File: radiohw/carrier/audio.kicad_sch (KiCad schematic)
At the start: 3 parts, among them U4 PCM2902, U5 PCM2902

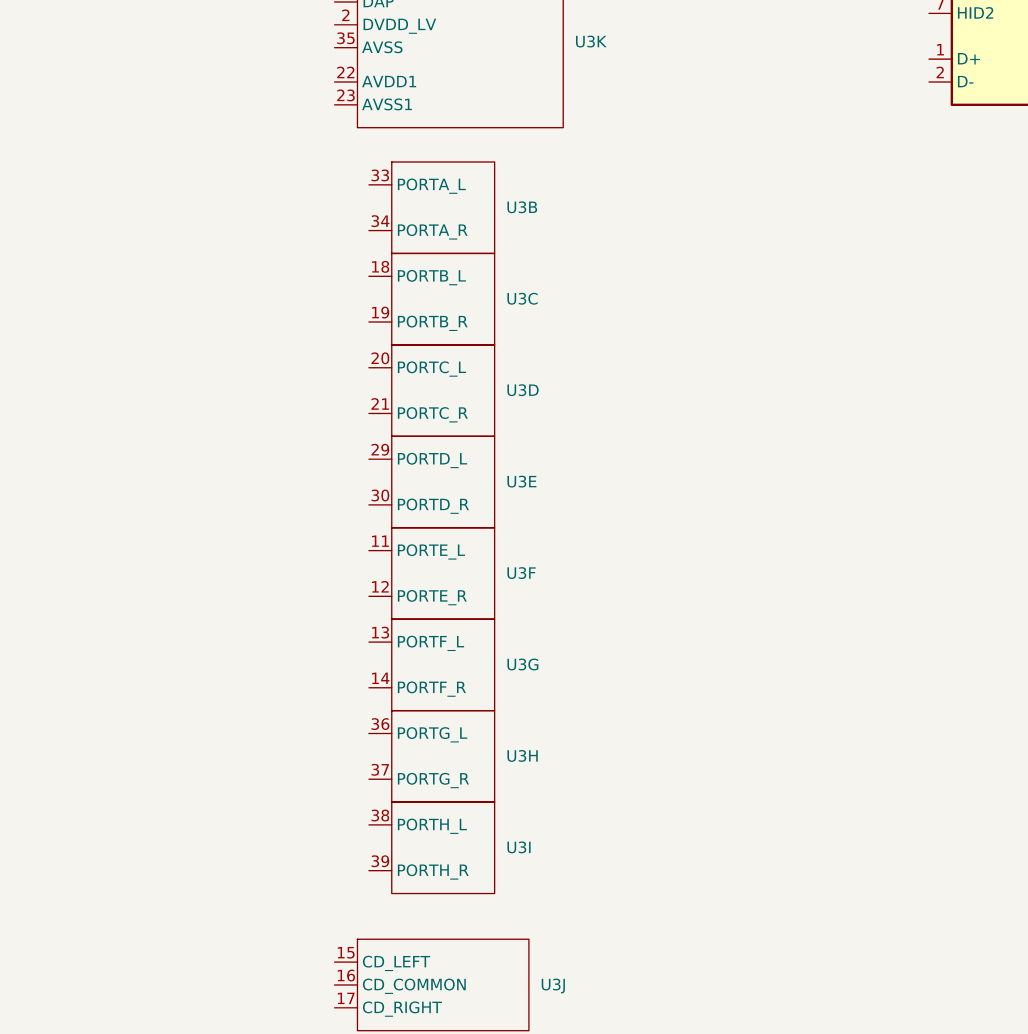
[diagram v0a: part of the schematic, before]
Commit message: Schematic development.
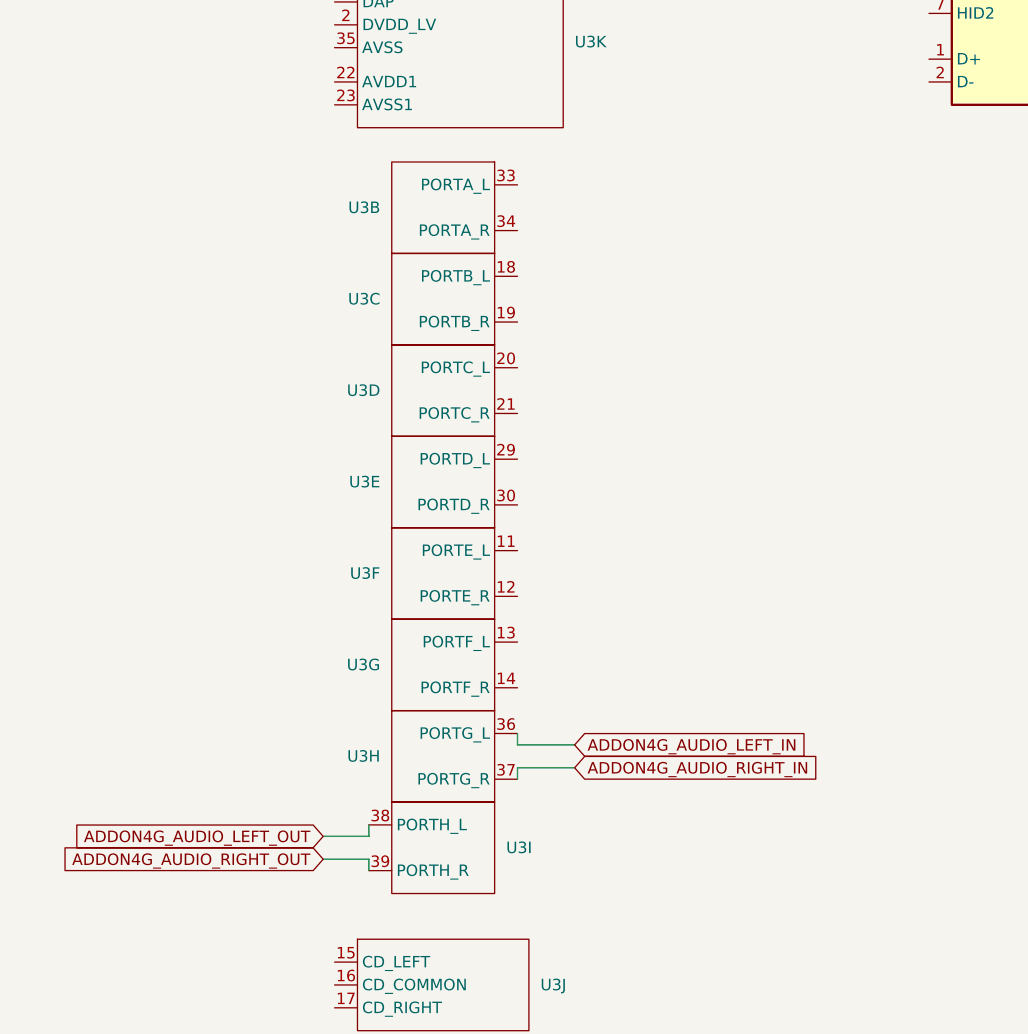
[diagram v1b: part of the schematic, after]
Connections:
- net ADDON4G_AUDIO_LEFT_OUT: now reaches U3.38 (PORTH_L)
- net ADDON4G_AUDIO_RIGHT_OUT: now reaches U3.39 (PORTH_R)
- net ADDON4G_AUDIO_LEFT_IN: now reaches U3.36 (PORTG_L)
- net ADDON4G_AUDIO_RIGHT_IN: now reaches U3.37 (PORTG_R)
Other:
- moved on the sheet: U3B, U3C, U3D, U3E, U3F, U3G, U3H

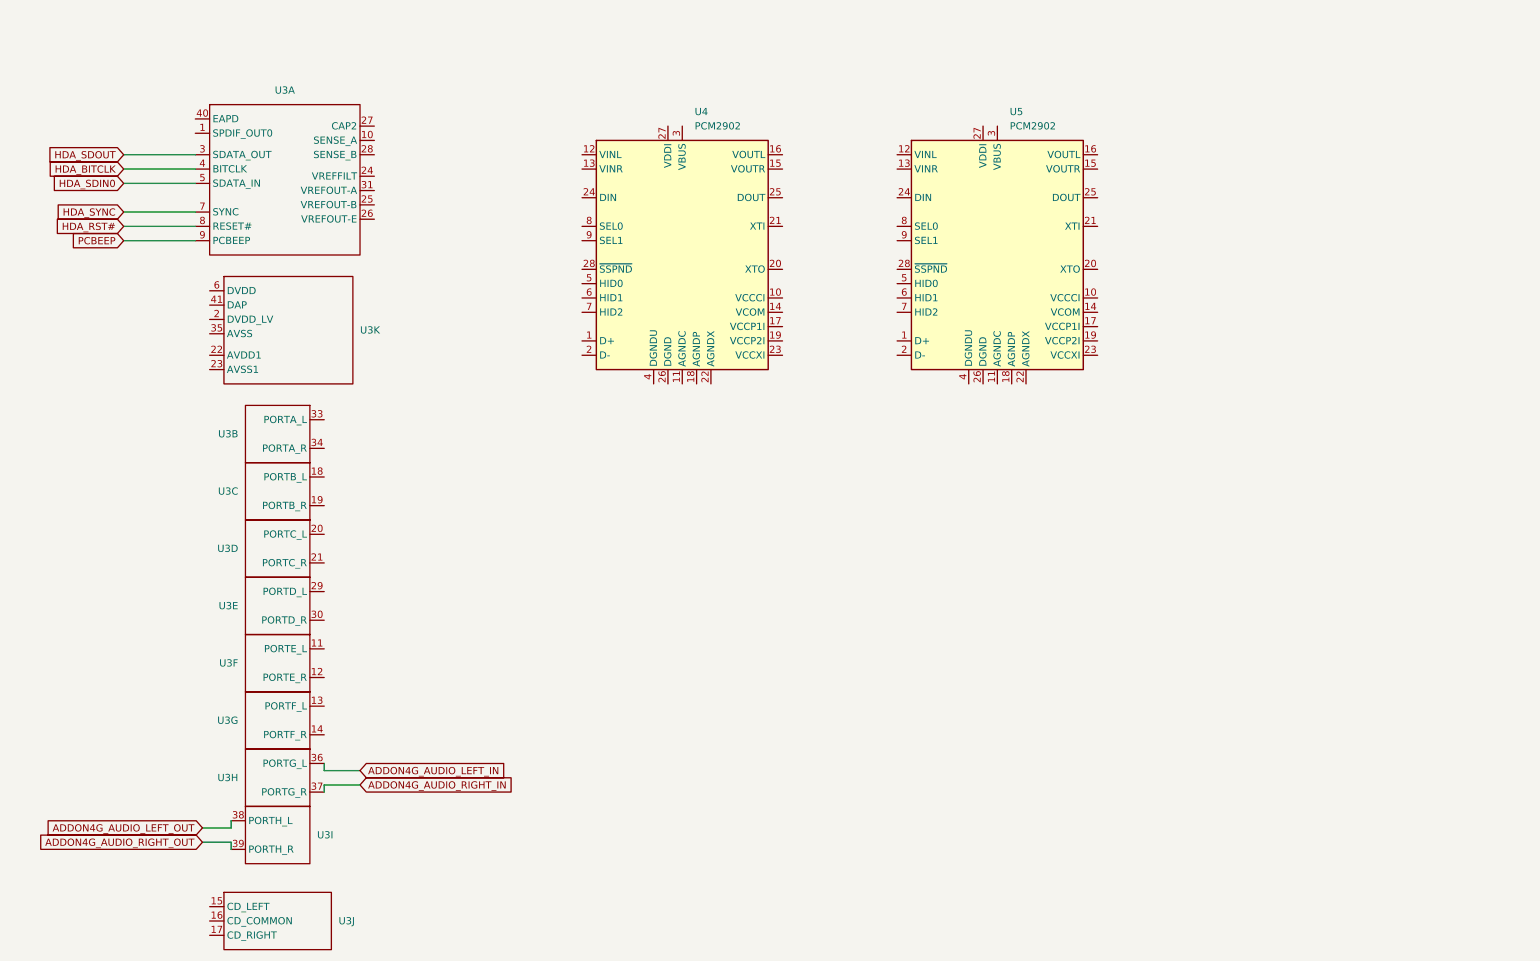
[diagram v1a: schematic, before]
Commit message: Schematic work.
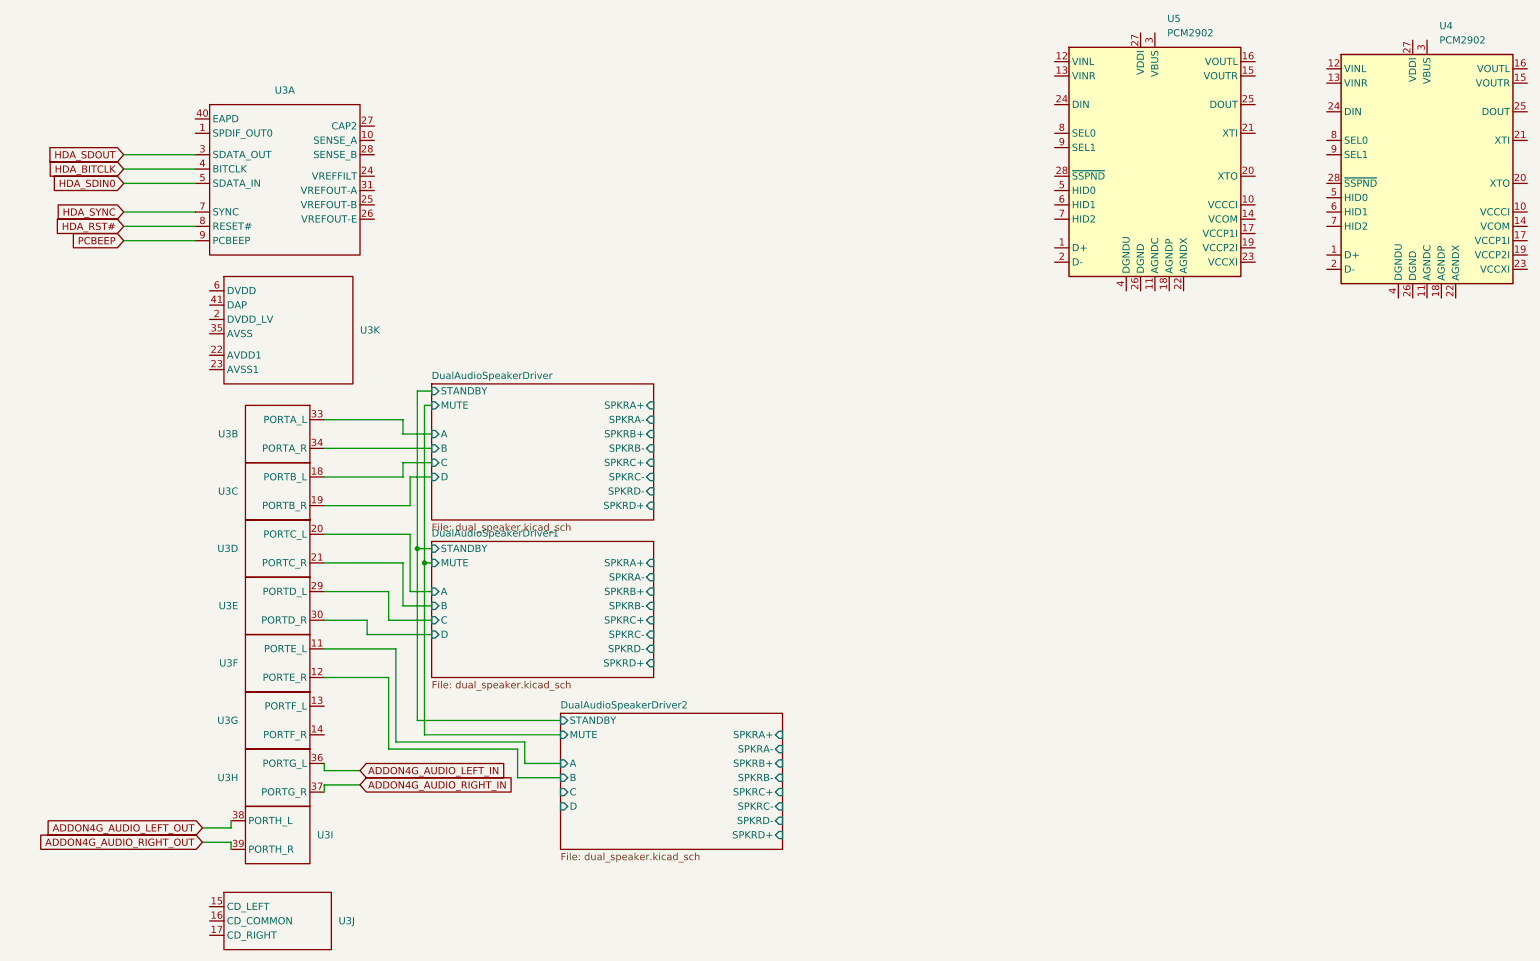
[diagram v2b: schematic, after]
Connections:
- net DualAudioSpeakerDriver1/C: now reaches U3.29 (PORTD_L)
- net DualAudioSpeakerDriver1/D: now reaches U3.30 (PORTD_R)
- net DualAudioSpeakerDriver2/A: now reaches U3.11 (PORTE_L)
- net DualAudioSpeakerDriver2/B: now reaches U3.12 (PORTE_R)
- net DualAudioSpeakerDriver/A: now reaches U3.33 (PORTA_L)
- net DualAudioSpeakerDriver/B: now reaches U3.34 (PORTA_R)
- net DualAudioSpeakerDriver1/A: now reaches U3.20 (PORTC_L)
- net DualAudioSpeakerDriver1/B: now reaches U3.21 (PORTC_R)
- net DualAudioSpeakerDriver/C: now reaches U3.18 (PORTB_L)
- net DualAudioSpeakerDriver/D: now reaches U3.19 (PORTB_R)
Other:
- added sheet DualAudioSpeakerDriver (dual_speaker.kicad_sch)
- added sheet DualAudioSpeakerDriver1 (dual_speaker.kicad_sch)
- added sheet DualAudioSpeakerDriver2 (dual_speaker.kicad_sch)
- moved on the sheet: U4, U5

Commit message: Audio schematic development.
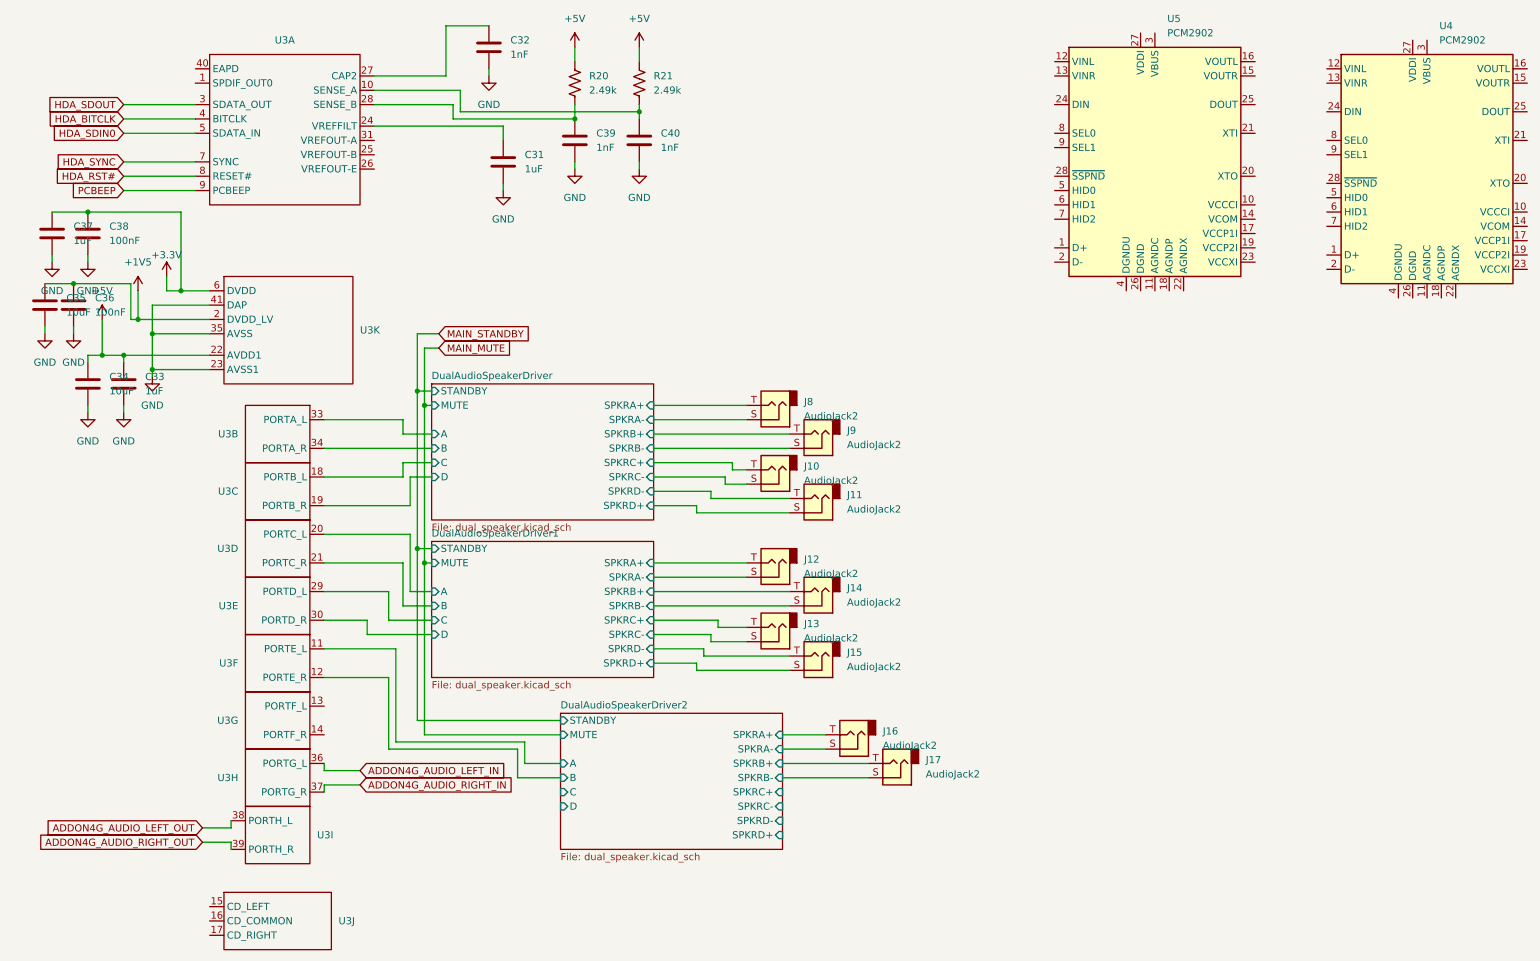
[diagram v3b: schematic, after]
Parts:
- added C31, C33, C37: 1uF, Capacitor_SMD:C_0805_2012Metric_Pad1.18x1.45mm_HandSolder, symbol Device:C
- added C32, C39, C40: 1nF, Capacitor_SMD:C_0402_1005Metric_Pad0.74x0.62mm_HandSolder, symbol Device:C
- added C34, C35: 10uF, symbol Device:C
- added C36, C38: 100nF, Capacitor_SMD:C_0603_1608Metric_Pad1.08x0.95mm_HandSolder, symbol Device:C
- added J10, J11, J12, J13, J14, J15, J16, J17, J8, J9: AudioJack2, symbol Connector_Audio:AudioJack2
- added R20, R21: 2.49k, Capacitor_SMD:C_0603_1608Metric_Pad1.08x0.95mm_HandSolder, symbol Device:R_US
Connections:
- net DualAudioSpeakerDriver/SPKRA+: now also J8.T
- net DualAudioSpeakerDriver/SPKRA-: now also J8.S
- net DualAudioSpeakerDriver/SPKRB+: now also J9.T
- net DualAudioSpeakerDriver/SPKRB-: now also J9.S
- net DualAudioSpeakerDriver/SPKRC+: now also J10.T
- net DualAudioSpeakerDriver/SPKRC-: now also J10.S
- net DualAudioSpeakerDriver/SPKRD+: now also J11.S
- net DualAudioSpeakerDriver/SPKRD-: now also J11.T
- net DualAudioSpeakerDriver1/SPKRA+: now also J12.T
- net DualAudioSpeakerDriver1/SPKRA-: now also J12.S
- net DualAudioSpeakerDriver1/SPKRB+: now also J14.T
- net DualAudioSpeakerDriver1/SPKRB-: now also J14.S
- net DualAudioSpeakerDriver1/SPKRC+: now also J13.T
- net DualAudioSpeakerDriver1/SPKRC-: now also J13.S
- net DualAudioSpeakerDriver1/SPKRD+: now also J15.S
- net DualAudioSpeakerDriver1/SPKRD-: now also J15.T
- net DualAudioSpeakerDriver2/SPKRA+: now also J16.T
- net DualAudioSpeakerDriver2/SPKRA-: now also J16.S
- net DualAudioSpeakerDriver2/SPKRB+: now also J17.T
- net DualAudioSpeakerDriver2/SPKRB-: now also J17.S
- net +1V5: now reaches U3.2 (DVDD_LV)
- net +1V5: now also C35.1, C36.1
- net +5V: now reaches U3.22 (AVDD1)
- net +5V: now also C33.1, C34.1, R20.1, R21.1
- net GND: now reaches U3.23 (AVSS1)
- net GND: now also U3.35 (AVSS), U3.41 (DAP), C31.2, C32.2, C33.2, C34.2, C35.2, C36.2, C37.2, C38.2, C39.2, C40.2
- net +3.3V: now reaches U3.6 (DVDD)
- net +3.3V: now also C37.1, C38.1
- net at U3.10 (SENSE_A): now also C40.1, R21.2
- net at U3.24 (VREFFILT): now also C31.1
- net at U3.27 (CAP2): now also C32.1
- net at U3.28 (SENSE_B): now also C39.1, R20.2
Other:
- moved on the sheet: U3A
